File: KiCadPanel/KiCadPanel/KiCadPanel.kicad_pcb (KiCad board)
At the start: 4 copper layers, 64 x 64 mm, 320 parts, among them IC1 STP16CPC26PTR, IC10 STP16CPC26PTR, IC11 74HC4514PW,118, IC12 AP2281-3WG-7, IC13 AP2281-3WG-7, IC14 AP2281-3WG-7, IC15 AP2281-3WG-7, IC16 STP16CPC26PTR, IC17 AP2281-3WG-7, IC18 AP2281-3WG-7, IC19 AP2281-3WG-7, IC2 AP2281-3WG-7, IC20 AP2281-3WG-7, IC3 AP2281-3WG-7, IC4 AP2281-3WG-7, IC5 AP2281-3WG-7, IC6 AP2281-3WG-7, IC7 AP2281-3WG-7, IC8 AP2281-3WG-7, IC9 AP2281-3WG-7, J1 15-91-0100

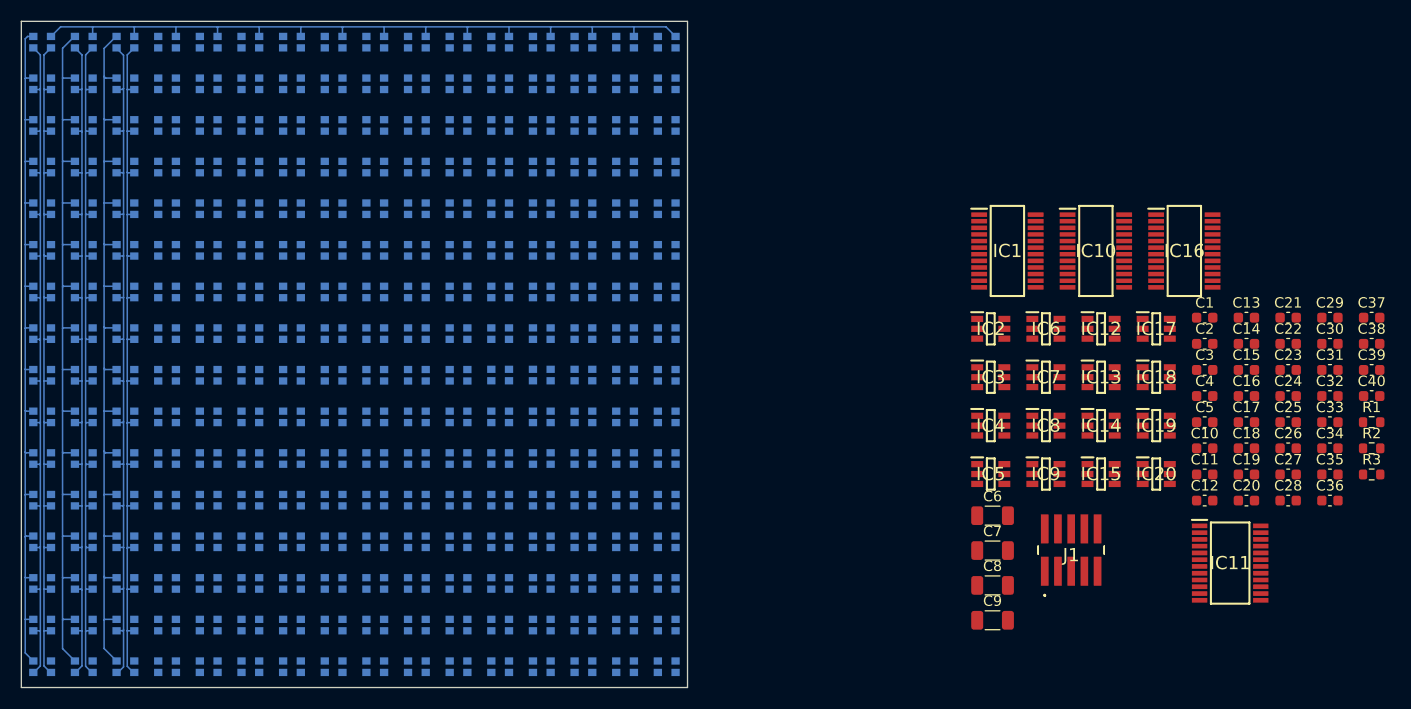
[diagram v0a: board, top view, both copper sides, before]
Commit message: Update for MTE
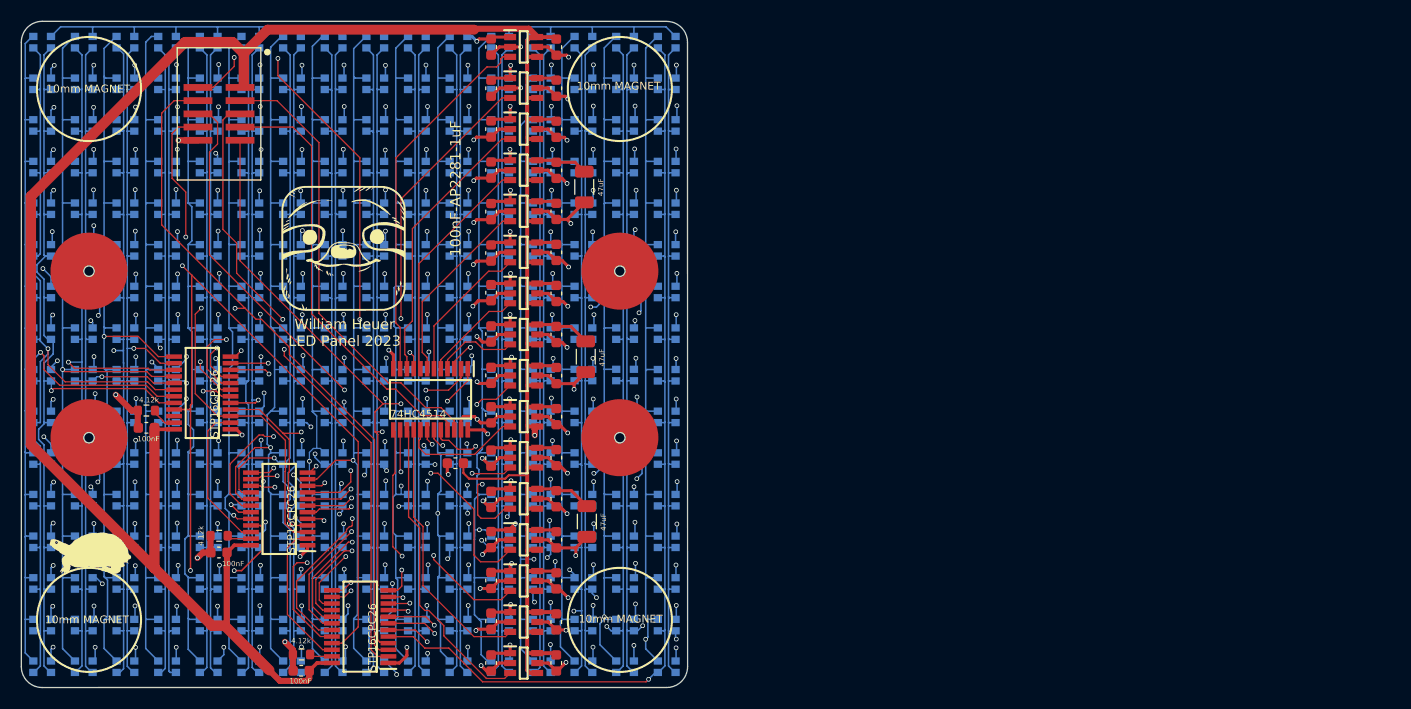
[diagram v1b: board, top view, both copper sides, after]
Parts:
- removed C9: 47u, Capacitor_SMD:C_1206_3216Metric
- added G***: LOGO, LOGO, F.Cu at (106.6, 101.1)
- added G***: LOGO, LOGO, F.Cu at (130.9, 71.8)
- added H100: MountingHole, Mounting_Wuerth:Mounting_Wuerth_WA-SMSE-ExternalM3_H5mm_9771050360, F.Cu at (157.5, 74.0)
- added H101: MountingHole, Mounting_Wuerth:Mounting_Wuerth_WA-SMSE-ExternalM3_H5mm_9771050360, F.Cu at (157.5, 90.0)
- added H102: MountingHole, Mounting_Wuerth:Mounting_Wuerth_WA-SMSE-ExternalM3_H5mm_9771050360, F.Cu at (106.5, 74.0)
- added H103: MountingHole, Mounting_Wuerth:Mounting_Wuerth_WA-SMSE-ExternalM3_H5mm_9771050360, F.Cu at (106.5, 90.0)
- J1: value 15-91-0100 -> ~; footprint SamacSys_Parts:FTSH10501FDVK -> LEDCubePanel:CNC_TECH_SMD_10POS
- moved R3 117.9 mm to (112.0, 87.4), turned to 180 degrees
- moved C32 113.7 mm to (112.0, 89.0), turned to 180 degrees
- moved R2 111.0 mm to (119.0, 99.4), turned to 180 degrees
- moved R1 105.2 mm to (126.9, 110.8), turned to 180 degrees
- moved C18 99.2 mm to (119.0, 101.0), turned to 180 degrees
- moved IC16 95.3 mm to (117.4, 85.7), turned to 180 degrees
- moved C1 93.2 mm to (126.9, 112.4), turned to 180 degrees
- moved J1 90.2 mm to (121.0, 58.9), turned to -90 degrees
- moved C40 88.4 mm to (145.1, 111.6), turned to -90 degrees
- moved C37 85.8 mm to (145.1, 64.3), turned to -90 degrees
- moved C39 85.5 mm to (145.1, 95.9), turned to -90 degrees
- moved C38 84.6 mm to (145.1, 80.0), turned to -90 degrees
- moved C28 84.5 mm to (145.1, 60.4), turned to -90 degrees
- moved C31 84.1 mm to (145.1, 107.6), turned to -90 degrees
- moved C20 82.7 mm to (145.1, 56.4), turned to -90 degrees
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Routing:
- net +3V3: track 0.00 -> 296.0 mm, vias 0 -> 2
- net GND: track 0.00 -> 144.1 mm, vias 0 -> 41
- net LED_4_GREEN: track 0.00 -> 104.4 mm, vias 0 -> 2
- net LED_3_GREEN: track 0.00 -> 103.7 mm, vias 0 -> 2
- net LED_0_GREEN: track 0.00 -> 103.0 mm, vias 0 -> 2
- net BRIGHTNESS_PWM: track 0.00 -> 102.0 mm, vias 0 -> 4
- net LED_4_BLUE: track 0.00 -> 101.7 mm, vias 0 -> 2
- net LED_3_BLUE: track 0.00 -> 99.6 mm, vias 0 -> 2
- net LED_0_BLUE: track 0.00 -> 99.5 mm, vias 0 -> 2
- net MASTER_CLK: track 0.00 -> 99.1 mm, vias 0 -> 2
- net LED_1_GREEN: track 0.00 -> 99.0 mm, vias 0 -> 2
- net LED_2_GREEN: track 0.00 -> 98.5 mm, vias 0 -> 2
- net LED_0_RED: track 0.00 -> 98.4 mm, vias 0 -> 1
- net LED_2_BLUE: track 0.00 -> 98.4 mm, vias 0 -> 2
- net LED_1_BLUE: track 0.00 -> 97.4 mm, vias 0 -> 2
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- added copper zone on In1.Cu, net GND
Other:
- outline, holes or cut-outs redrawn
- board text added: "100nF"
- board text added: "100nF-AP2281-1uF"
- board text added: "10mm MAGNET"
- board text added: "4.12k"
- board text added: "47uF"
- board text added: "74HC4514"
- board text added: "STP16CPC26"
- board text added: "William Heuer LED Panel 2023"
